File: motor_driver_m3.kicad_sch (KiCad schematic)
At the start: 50 parts, among them J7 Conn_01x01_Pin, J8 Conn_01x01_Pin, J9 Conn_01x01_Pin, M3 STM32C011F6U6TR, Q13 NP80N06D6, Q14 NP80N06D6, Q15 NP80N06D6, Q16 NP80N06D6, Q17 NP80N06D6, Q18 NP80N06D6

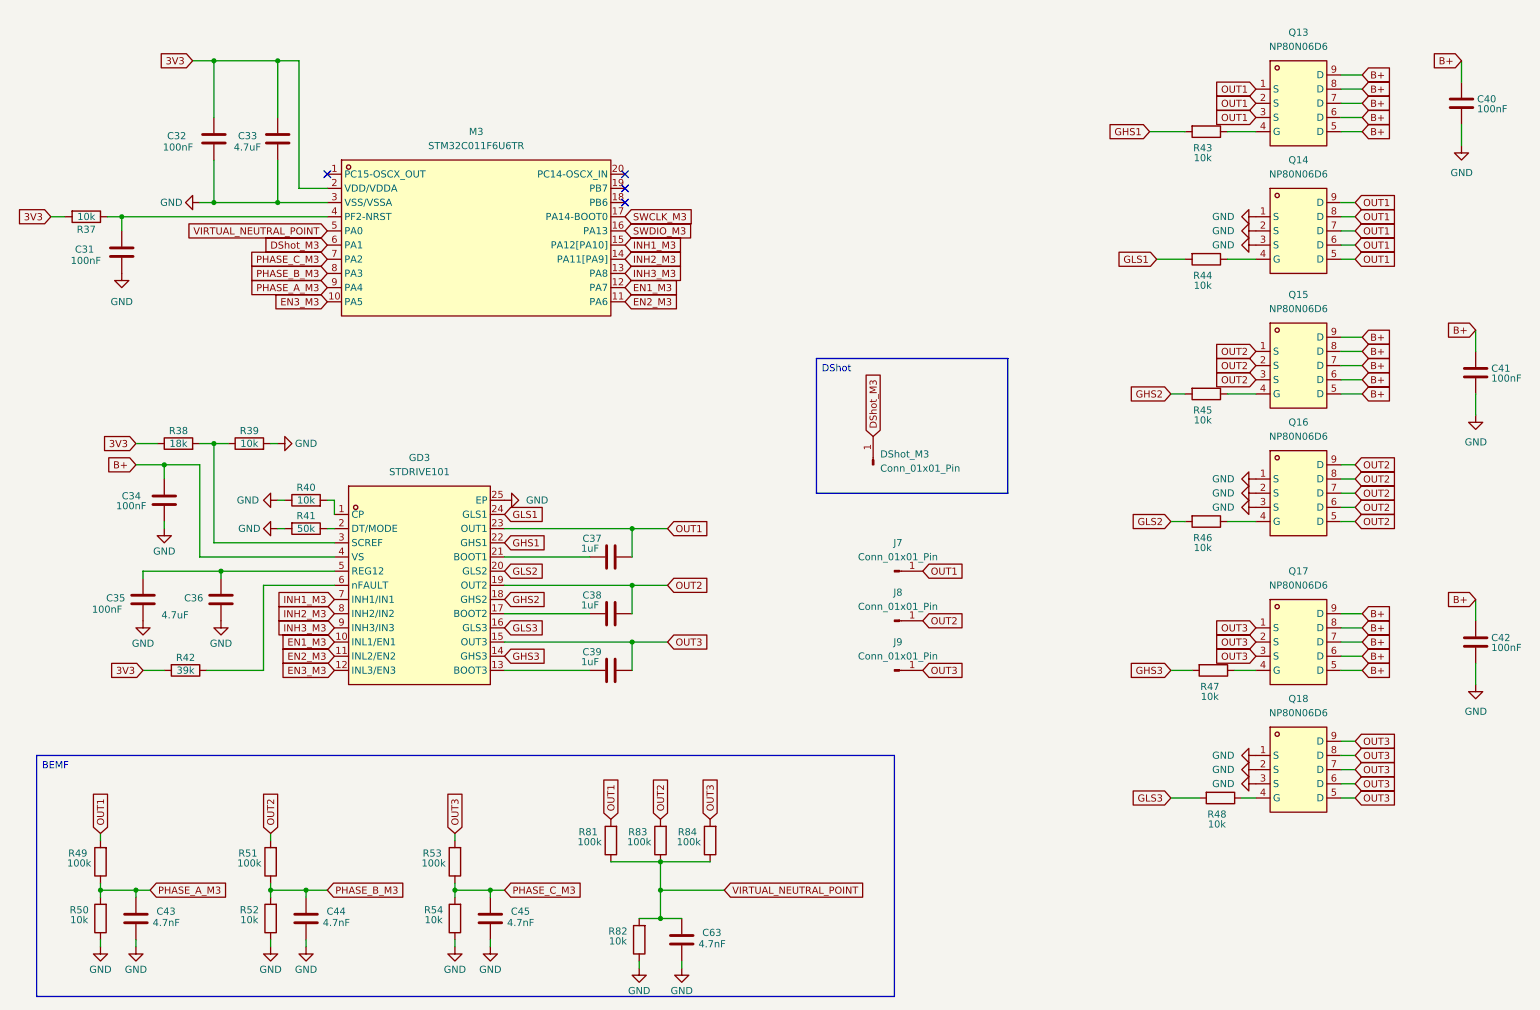
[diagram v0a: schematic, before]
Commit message: ...
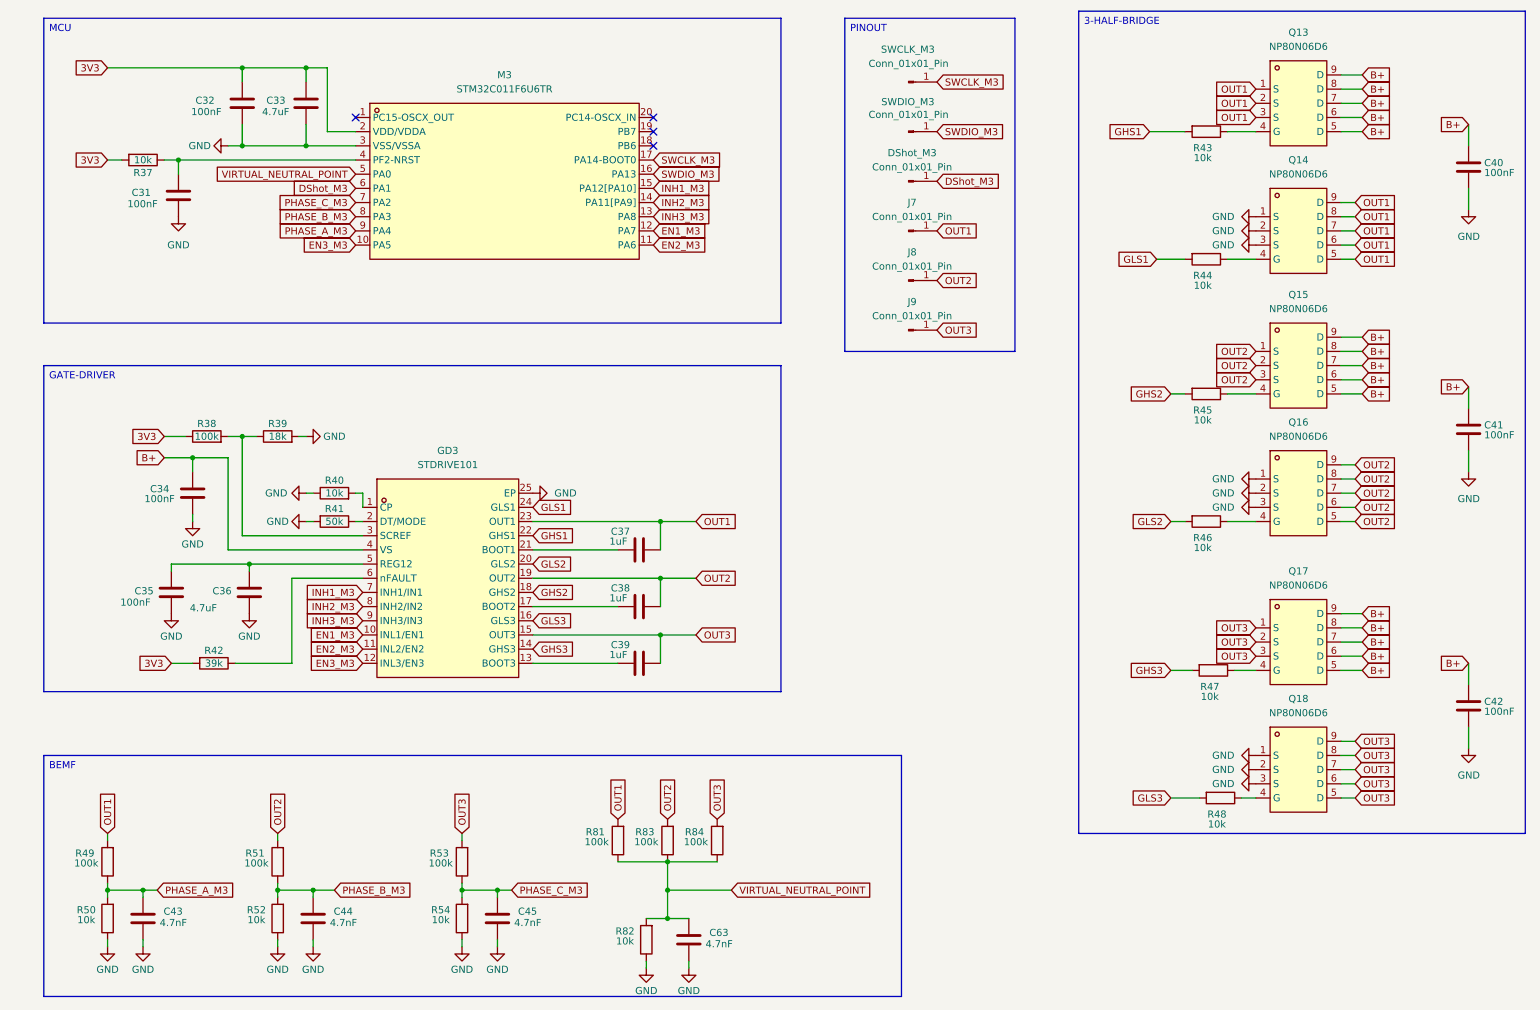
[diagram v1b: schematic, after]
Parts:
- added SWCLK_M3, SWDIO_M3: Conn_01x01_Pin, deshan:Conn_01x01_Pin, symbol Connector:Conn_01x01_Pin
- R38: value 18k -> 100k
- R39: value 10k -> 18k
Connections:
- net SWCLK_M3: now also SWCLK_M3.1 (Pin_1)
- net SWDIO_M3: now also SWDIO_M3.1 (Pin_1)
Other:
- moved on the sheet: C31, C32, C33, C34, C35, C36, C37, C38, C39, C40, C41, C42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
